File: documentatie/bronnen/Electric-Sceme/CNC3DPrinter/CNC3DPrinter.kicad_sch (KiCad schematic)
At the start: 5 parts, among them M1 Stepper_Motor_bipolar, U1 Rotary Encoder 600R/P

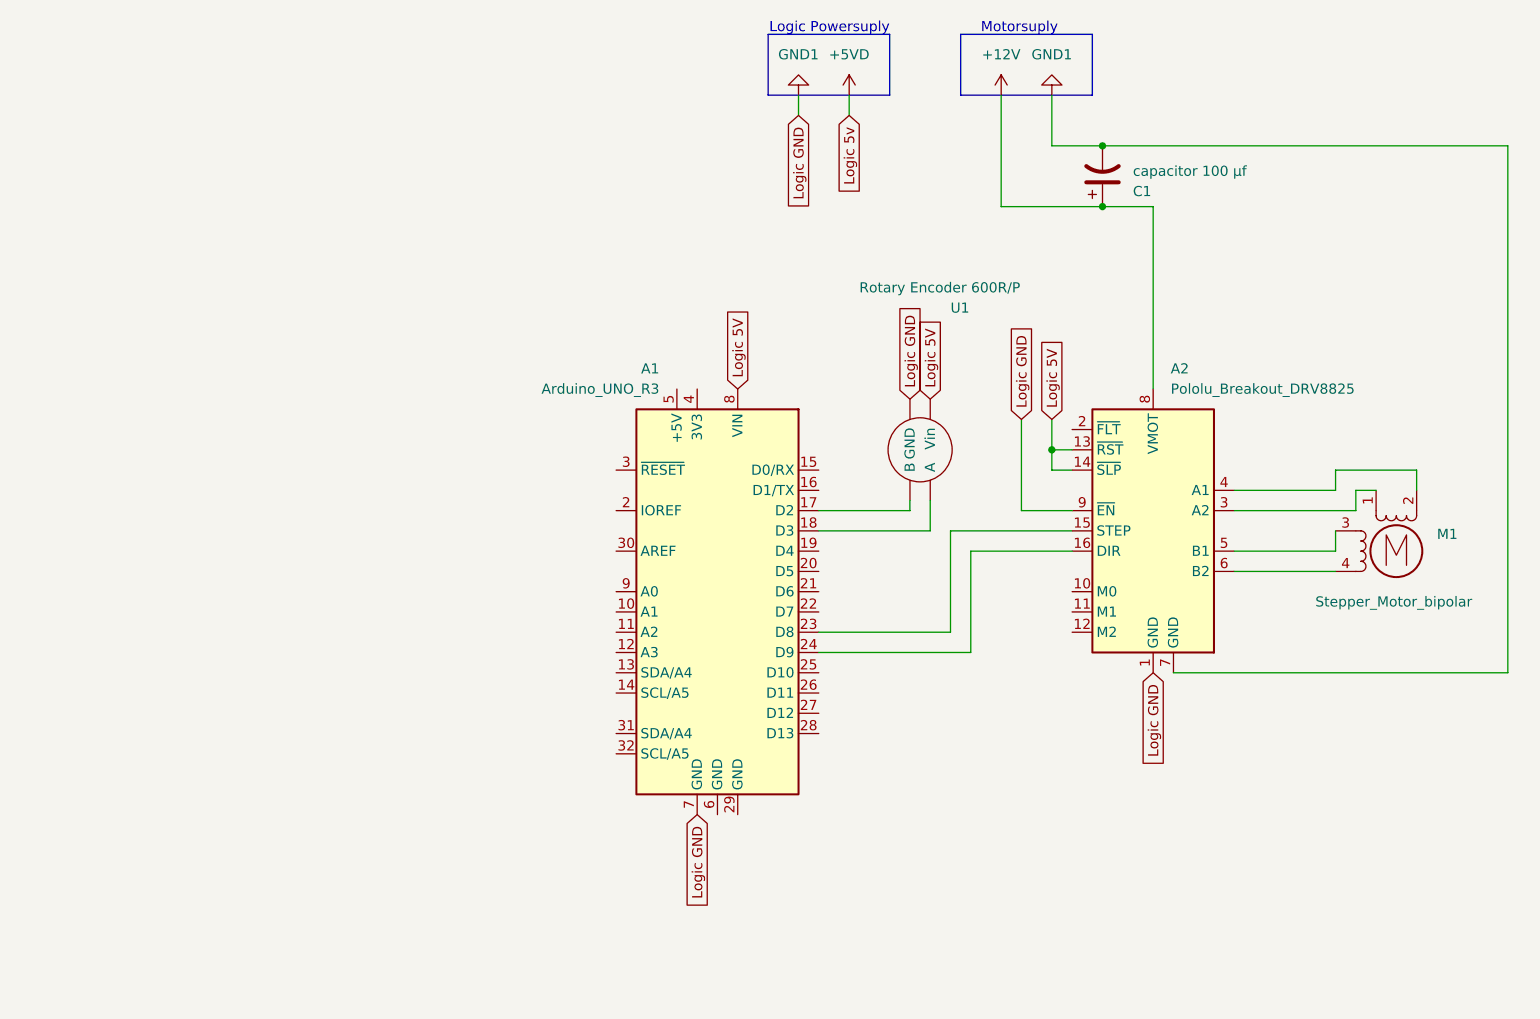
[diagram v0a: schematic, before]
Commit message: .
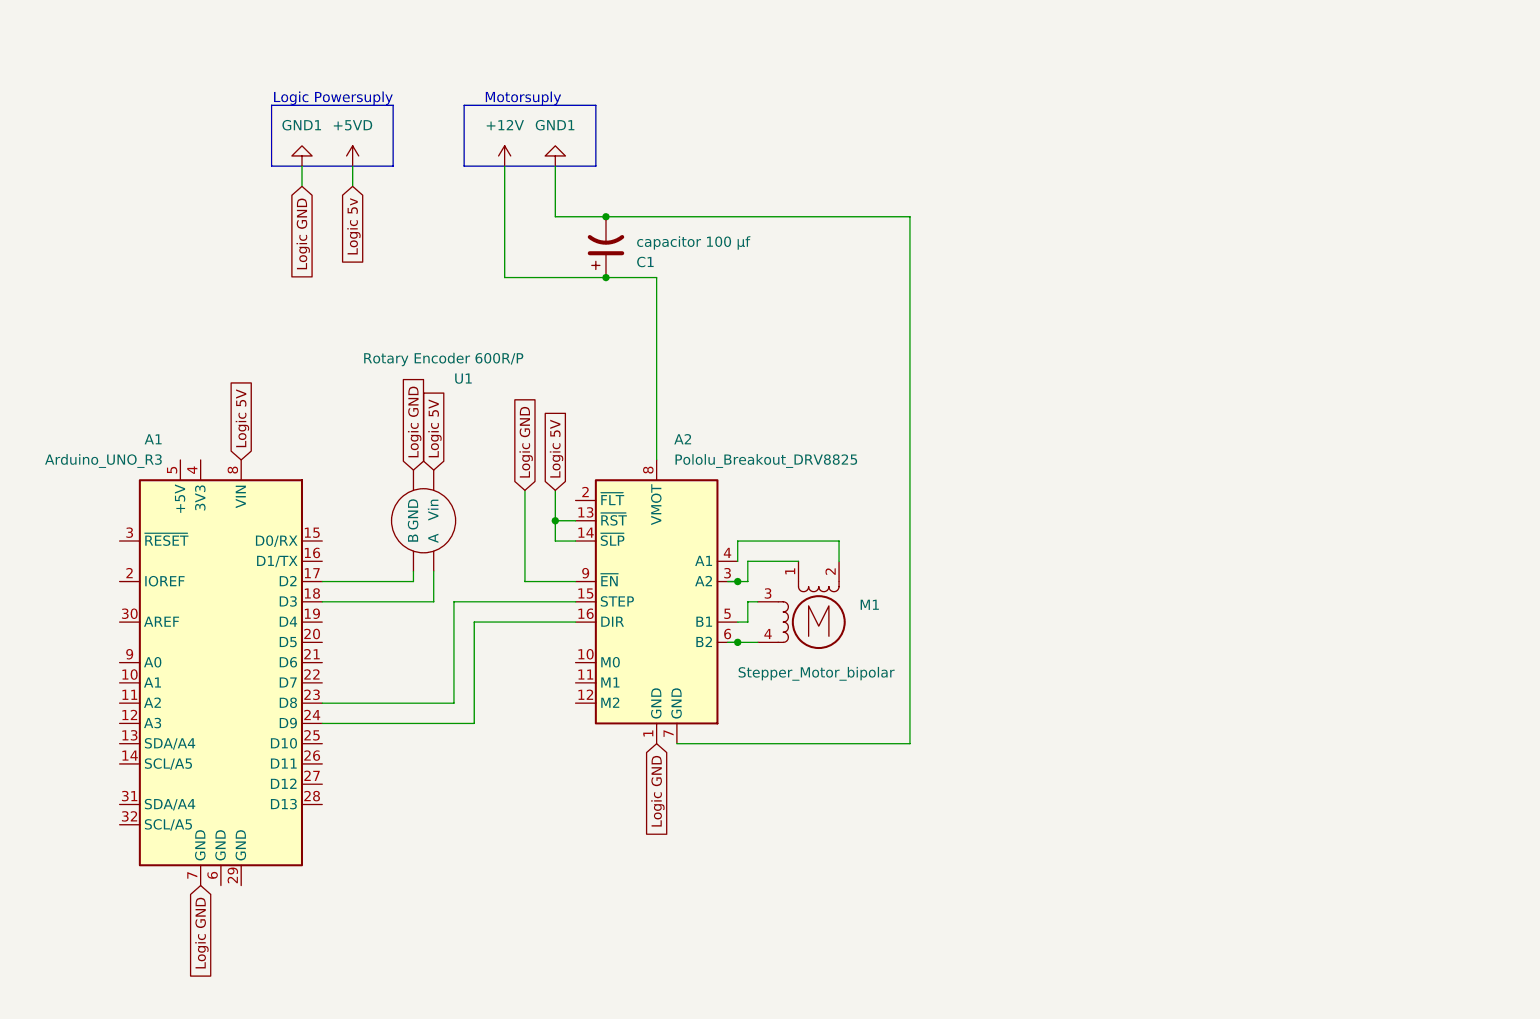
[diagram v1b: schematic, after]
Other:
- company: (none) -> Sens2Sea
- title: (none) -> Elektrisch schema 1 as
- moved on the sheet: A1, A2, C1, M1, U1
